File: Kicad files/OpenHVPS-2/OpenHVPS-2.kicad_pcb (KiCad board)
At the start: 2 copper layers, 47.1 x 20.5 mm, 67 parts, among them J1 Conn_01x03_Male, J2 Conn_01x03_Male, Q1 FQT7N10, Q2 BC846, Q3 MMDT3906, U1 74HC14, U2 MAX4162, U3 CD14538BM, U4 MAX6008AEUR+T

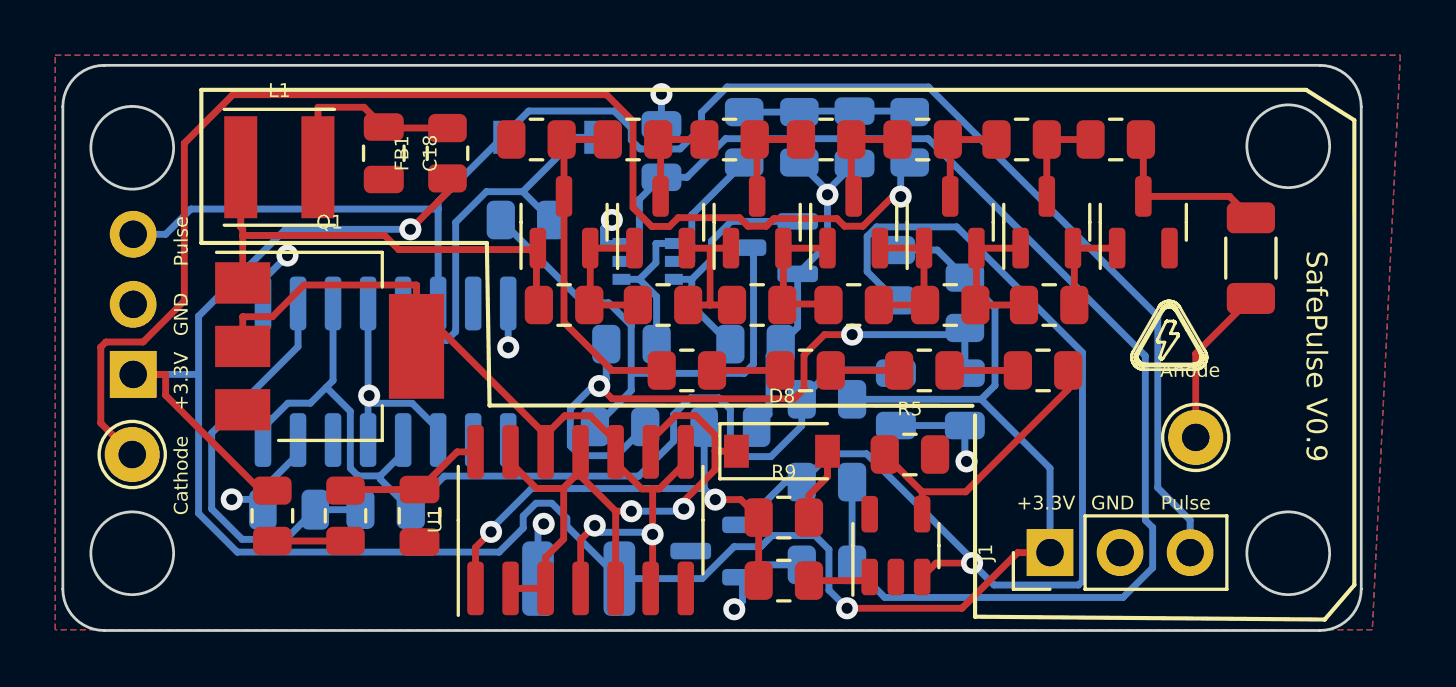
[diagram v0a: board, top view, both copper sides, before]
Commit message: small changes board layout and rerouted
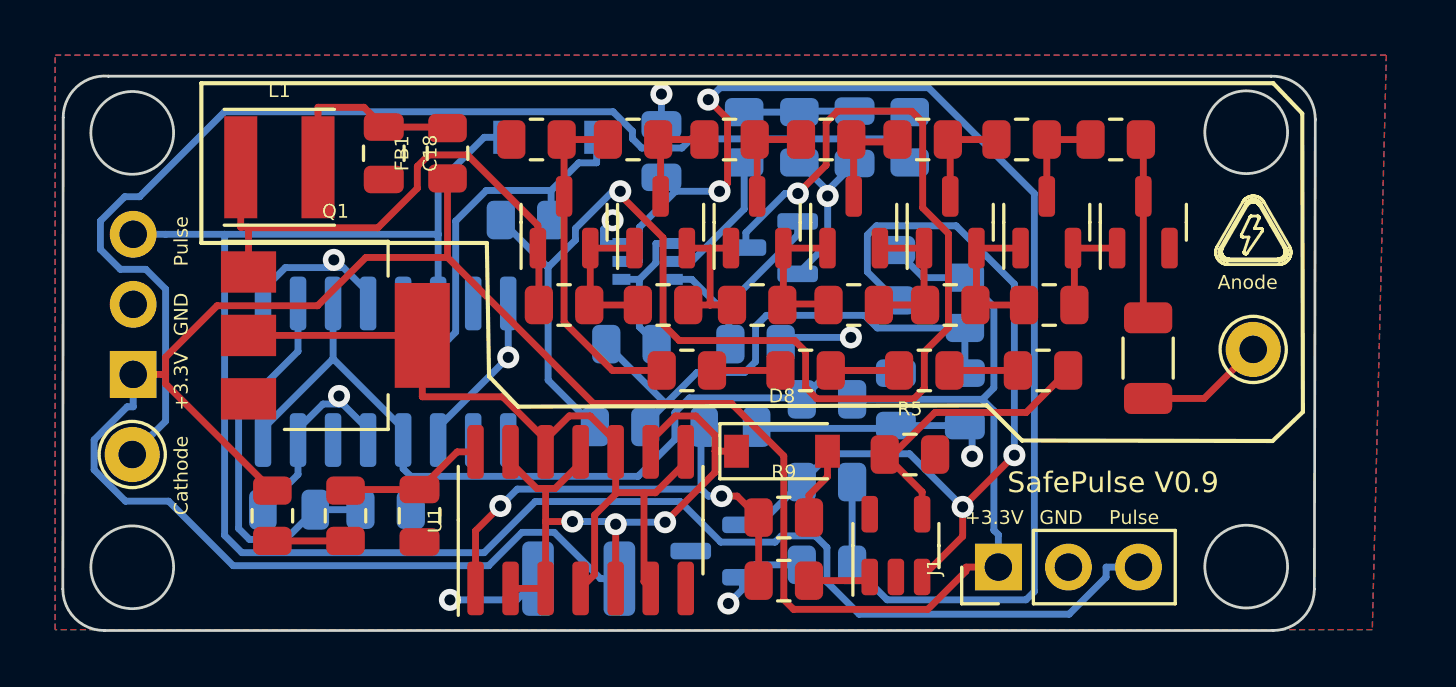
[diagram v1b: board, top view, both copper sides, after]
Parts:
- moved R7 5.20 mm to (160.3, 67.6)
- moved H5 3.81 mm to (164.1, 67.3)
- moved J1 1.95 mm to (154.8, 75.2)
- moved Q1 0.45 mm to (130.8, 66.8)
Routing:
- net Net-(Q2-Pad3): track 19.4 -> 50.1 mm, vias 0 -> 2
- net +3V3: track 84.6 -> 96.1 mm, vias 2 -> 0
- net Net-(D9-Pad2): track 57.3 -> 67.2 mm
- net +2V5: track 38.4 -> 31.0 mm, vias 1 -> 2
- net GND: track 40.8 -> 46.7 mm
- net Net-(C21-Pad1): track 24.4 -> 18.9 mm, vias 2 -> 0
- net Net-(C19-Pad1): track 37.7 -> 32.5 mm
- net Net-(H2-Pad1): track 46.6 -> 42.7 mm, vias 1 -> 0
- net Net-(Q1-Pad2): track 33.4 -> 30.2 mm, vias 2 -> 0
- net Net-(C2-Pad1): track 17.2 -> 20.1 mm
- net Net-(H5-Pad1): track 5.87 -> 4.55 mm
- net Net-(C16-Pad1): track 15.0 -> 14.1 mm
- net Net-(Q2-Pad1): track 8.68 -> 7.87 mm
- net Net-(D8-Pad1): track 24.0 -> 23.8 mm, vias 2 -> 3
- net Net-(C20-Pad1): track 48.0 -> 48.1 mm, vias 0 -> 2
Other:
- board size 47.1 x 20.5 mm -> 45.4 x 20.1 mm
